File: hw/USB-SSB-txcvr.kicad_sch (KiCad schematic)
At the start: 0 parts

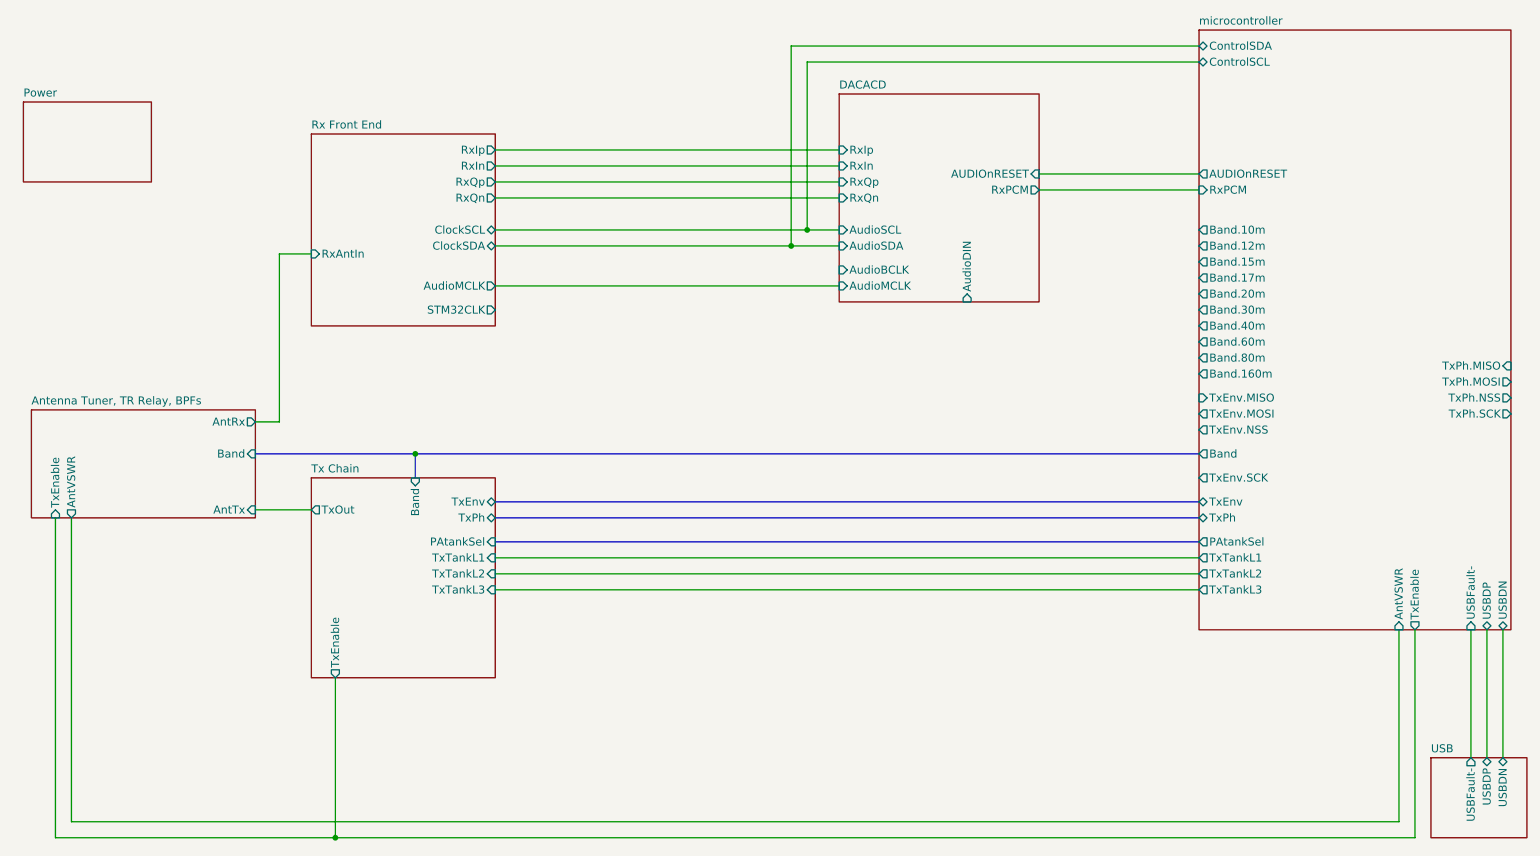
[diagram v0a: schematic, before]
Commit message: Checkpoint
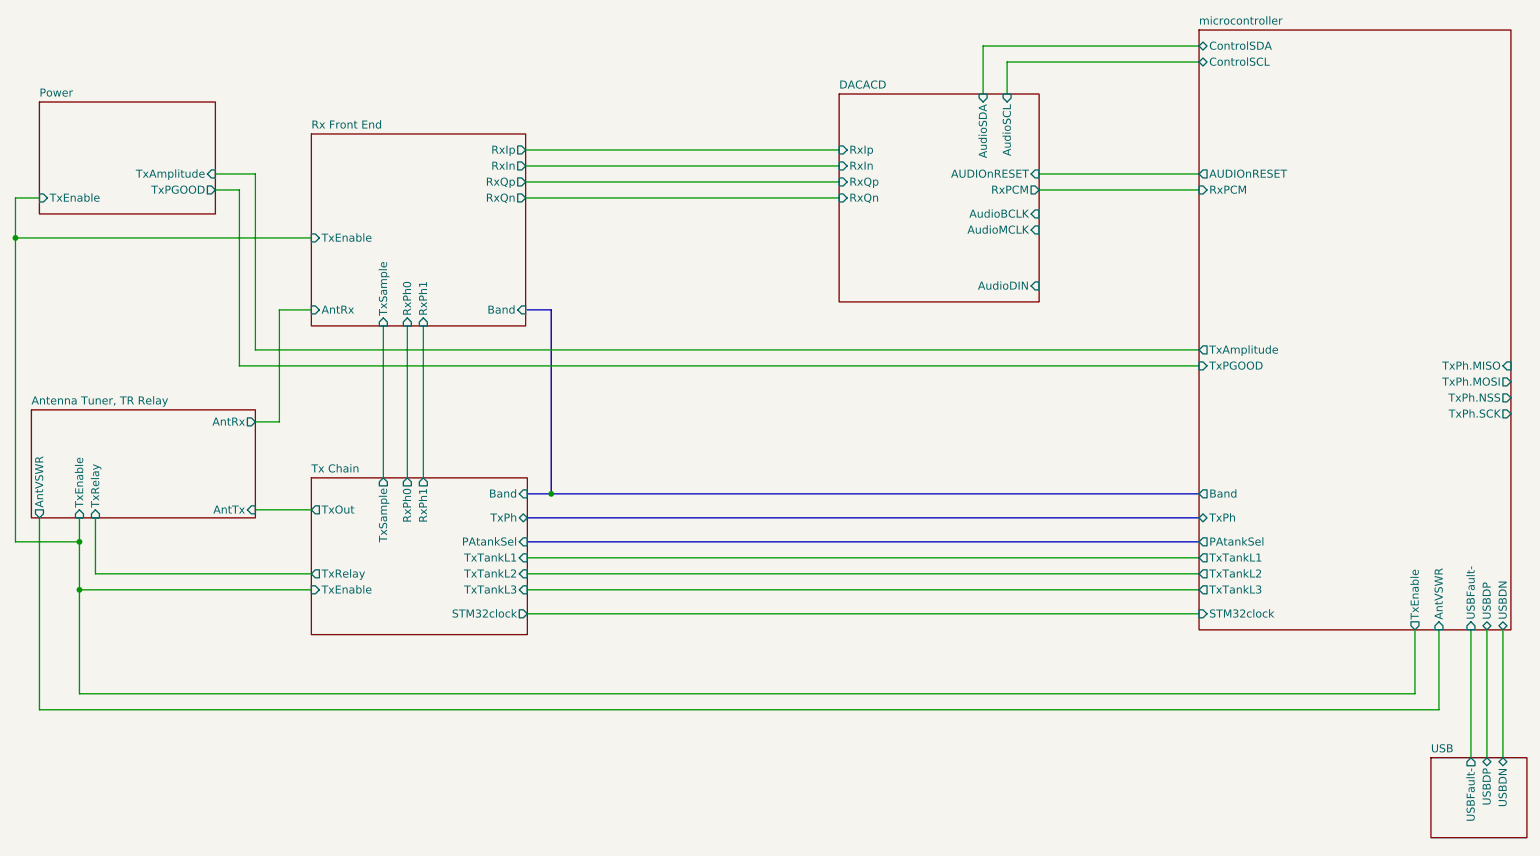
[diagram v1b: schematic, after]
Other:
- sheet Antenna Tuner, TR Relay, BPFs renamed Antenna Tuner, TR Relay
- sheet Antenna Tuner, TR Relay ports: added TxRelay; removed Band
- sheet Power ports: added TxAmplitude, TxEnable, TxPGOOD; removed none
- sheet Rx Front End ports: added AntRx, Band, RxPh0, RxPh1, TxEnable, TxSample; removed AudioMCLK, ClockSCL, ClockSDA, RxAntIn, STM32CLK
- sheet Tx Chain ports: added RxPh0, RxPh1, STM32clock, TxRelay, TxSample; removed TxEnv
- sheet microcontroller ports: added STM32clock, TxAmplitude, TxPGOOD; removed Band.10m, Band.12m, Band.15m, Band.160m, Band.17m, Band.20m, Band.30m, Band.40m, Band.60m, Band.80m, TxEnv, TxEnv.MISO, TxEnv.MOSI, TxEnv.NSS, TxEnv.SCK
